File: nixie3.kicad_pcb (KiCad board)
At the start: 2 copper layers, 153 x 96.5 mm, 64 parts, among them J1 AVR-ISP-10, J2 Barrel_Jack, J3 Conn_01x02_Pin, J4 Conn_01x02_Pin, J5 Conn_01x02_Pin, J6 Conn_01x02_Pin, J7 Conn_01x02_Pin, J8 Conn_01x02_Pin, Q1 IRFB4020PBF, U1 ATmega328-A, U2 MCP1401T-E/OT, U3 HV5222PG-G, U4 HV5222PG-G, U5 MC34063AP, Y1 10MHz / 12pF

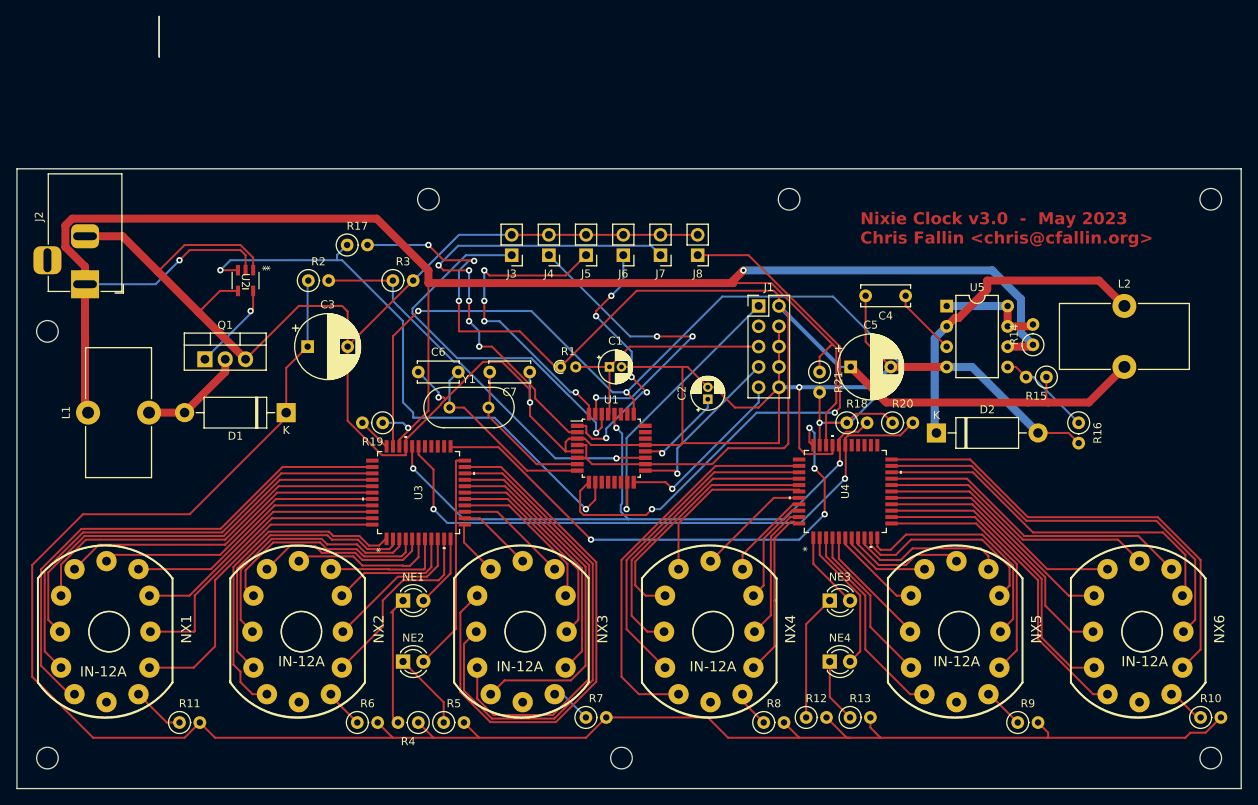
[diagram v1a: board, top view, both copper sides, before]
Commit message: board update
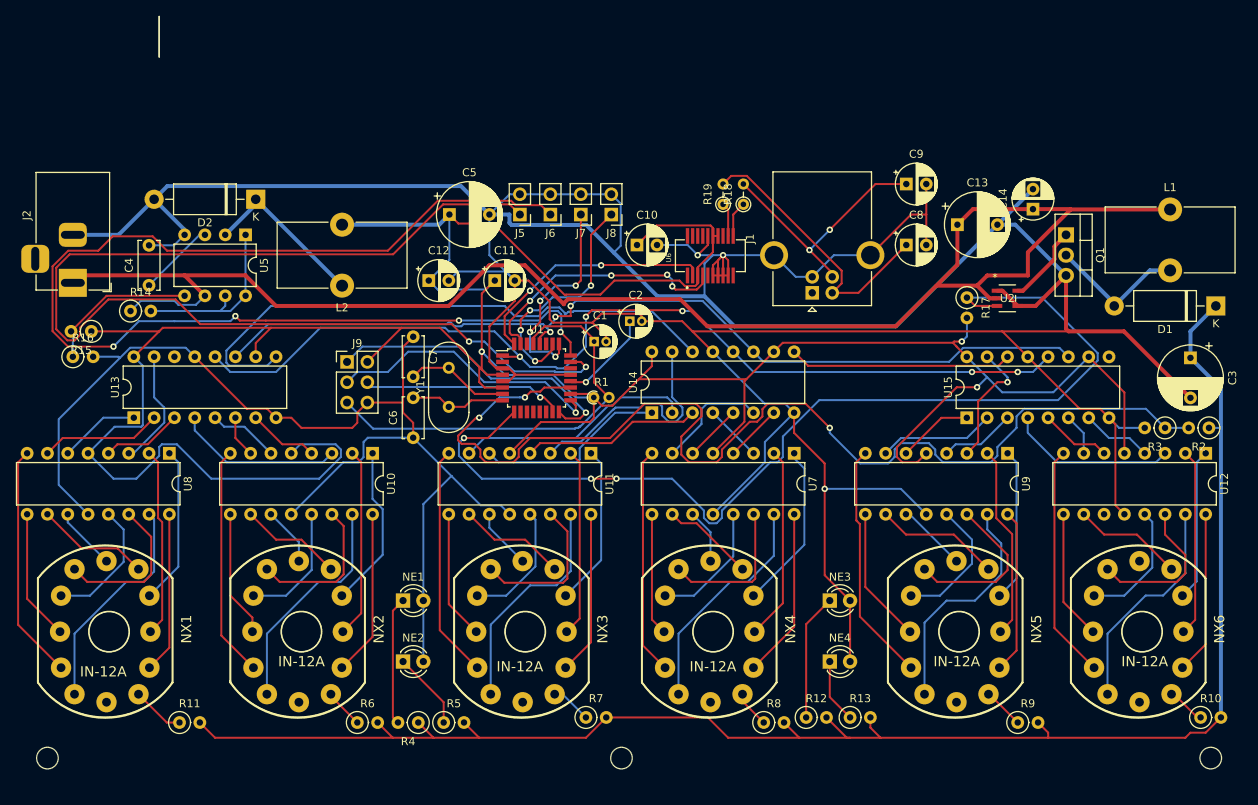
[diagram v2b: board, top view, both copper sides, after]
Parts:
- removed J3, J4: Conn_01x02_Pin, Connector_PinHeader_2.54mm:PinHeader_1x02_P2.54mm_Vertical
- removed R20, R21: 10k, Resistor_THT:R_Axial_DIN0207_L6.3mm_D2.5mm_P2.54mm_Vertical
- removed the REF** at (189.9, 38.7)
- removed the REF** at (44.5, 55.2)
- removed the REF** at (137.2, 38.7)
- removed the REF** at (92.1, 38.7)
- removed U3, U4: HV5222PG-G, import1:QFP44_10x10MC_MCH-M
- added C10: 100nF, Capacitor_THT:CP_Radial_D5.0mm_P2.50mm, F.Cu at (118.2, 44.5)
- added C11: 100nF, Capacitor_THT:CP_Radial_D5.0mm_P2.50mm, F.Cu at (100.4, 48.9)
- added C12: 10uF, Capacitor_THT:CP_Radial_D5.0mm_P2.50mm, F.Cu at (92.1, 48.9)
- added C13: 100uF 25V, Capacitor_THT:CP_Radial_D8.0mm_P5.00mm, F.Cu at (158.2, 41.9)
- added C14: 100nF, Capacitor_THT:CP_Radial_D5.0mm_P2.50mm, F.Cu at (167.6, 40.0)
- added C8: 47pF, Capacitor_THT:CP_Radial_D5.0mm_P2.50mm, F.Cu at (151.8, 44.5)
- added C9: 47pF, Capacitor_THT:CP_Radial_D5.0mm_P2.50mm, F.Cu at (151.8, 36.8)
- added J9: AVR-ISP-6, Connector_PinHeader_2.54mm:PinHeader_2x03_P2.54mm_Vertical, F.Cu at (81.9, 59.1)
- added U10: 74141, Package_DIP:DIP-16_W7.62mm, F.Cu at (85.1, 70.5)
- added U11: 74141, Package_DIP:DIP-16_W7.62mm, F.Cu at (112.4, 70.5)
- added U12: 74141, Package_DIP:DIP-16_W7.62mm, F.Cu at (189.2, 70.5)
- added U13: 74AHC595, Package_DIP:DIP-16_W7.62mm, F.Cu at (55.2, 66.0)
- added U14: 74HC595, Package_DIP:DIP-16_W7.62mm, F.Cu at (120.0, 65.4)
- added U15: 74HC595, Package_DIP:DIP-16_W7.62mm, F.Cu at (159.4, 66.0)
- added U6: FT231XS-R, import3:SOP63P599X175-20N, F.Cu at (127.3, 45.8)
- added U7: 74141, Package_DIP:DIP-16_W7.62mm, F.Cu at (137.8, 70.5)
- added U8: 74141, Package_DIP:DIP-16_W7.62mm, F.Cu at (59.7, 70.5)
- added U9: 74141, Package_DIP:DIP-16_W7.62mm, F.Cu at (164.5, 70.5)
- C3: value C -> 10uF 400V
- J1: value AVR-ISP-10 -> USB_B; footprint Connector_PinHeader_2.54mm:PinHeader_2x05_P2.54mm_Vertical -> Connector_USB:USB_B_OST_USB-B1HSxx_Horizontal
- J2: value Barrel_Jack -> 12V PWR
- R18, R19: value 10k -> 27; footprint Resistor_THT:R_Axial_DIN0207_L6.3mm_D2.5mm_P2.54mm_Vertical -> Resistor_THT:R_Axial_DIN0204_L3.6mm_D1.6mm_P2.54mm_Vertical
- moved L1 137.6 mm to (184.8, 40.0), turned to 0 degrees
- moved R16 126.0 mm to (47.6, 58.4), turned to 0 degrees
- moved R15 119.5 mm to (49.9, 55.2)
- moved D1 117.0 mm to (190.5, 52.1)
- moved R2 114.1 mm to (189.6, 67.3), turned to 180 degrees
- moved R14 112.9 mm to (54.8, 52.7), turned to 0 degrees
- moved C3 110.4 mm to (187.3, 58.6), turned to -90 degrees
- moved Q1 108.8 mm to (171.8, 43.2), turned to -90 degrees
- moved R3 98.3 mm to (184.2, 67.3), turned to 180 degrees
- moved L2 97.8 mm to (81.3, 49.5), turned to 180 degrees
- moved U2 95.3 mm to (164.4, 51.1), turned to 0 degrees
- moved C4 94.6 mm to (57.1, 49.5), turned to 90 degrees
- moved D2 90.0 mm to (70.5, 38.7), turned to 180 degrees
- moved U5 88.1 mm to (69.2, 43.2), turned to -90 degrees
- moved R17 77.7 mm to (159.4, 51.0), turned to -90 degrees
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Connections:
- C1 pad 1: Net-(J1-~{RST}) -> Net-(J9-~{RST})
- J1 pad 1: Net-(J1-MOSI) -> unconnected-(J1-VBUS-Pad1)
- J1 pad 2: VDD -> Net-(J1-D-)
- J1 pad 3: unconnected-(J1-NC-Pad3) -> Net-(J1-D+)
- J1 pad 5: Net-(J1-~{RST}) -> GND
- NE1 pad 2: /Net-(U3A-HVOUT12) -> GND
- NE2 pad 2: /Net-(U3A-HVOUT1) -> GND
- NE3 pad 2: /unconnected-(U4A-HVOUT22-Pad1) -> GND
- NE4 pad 2: /unconnected-(U4A-HVOUT21-Pad2) -> GND
- NX4 pad 0: /unconnected-(U4A-HVOUT23-Pad44) -> Net-(U7-~{Q0})
- NX4 pad 1: /unconnected-(U4A-HVOUT32-Pad35) -> Net-(U7-~{Q1})
- NX4 pad 2: /unconnected-(U4A-HVOUT31-Pad36) -> Net-(U7-~{Q2})
- NX4 pad 3: /unconnected-(U4A-HVOUT30-Pad37) -> Net-(U7-~{Q3})
- NX4 pad 4: /unconnected-(U4A-HVOUT29-Pad38) -> Net-(U7-~{Q4})
- NX4 pad 5: /unconnected-(U4A-HVOUT28-Pad39) -> Net-(U7-~{Q5})
- NX4 pad 6: /unconnected-(U4A-HVOUT27-Pad40) -> Net-(U7-~{Q6})
- NX4 pad 7: /unconnected-(U4A-HVOUT26-Pad41) -> Net-(U7-~{Q7})
- NX4 pad 8: /unconnected-(U4A-HVOUT25-Pad42) -> Net-(U7-~{Q8})
- NX4 pad 9: /unconnected-(U4A-HVOUT24-Pad43) -> Net-(U7-~{Q9})
- NX5 pad 0: /unconnected-(U4A-HVOUT11-Pad12) -> Net-(U9-~{Q0})
- NX5 pad 1: /unconnected-(U4A-HVOUT20-Pad3) -> Net-(U9-~{Q1})
- NX5 pad 2: /unconnected-(U4A-HVOUT19-Pad4) -> Net-(U9-~{Q2})
- NX5 pad 3: /unconnected-(U4A-HVOUT18-Pad5) -> Net-(U9-~{Q3})
- NX5 pad 4: /unconnected-(U4A-HVOUT17-Pad6) -> Net-(U9-~{Q4})
- NX5 pad 5: /unconnected-(U4A-HVOUT16-Pad7) -> Net-(U9-~{Q5})
- NX5 pad 6: /unconnected-(U4A-HVOUT15-Pad8) -> Net-(U9-~{Q6})
- NX5 pad 7: /unconnected-(U4A-HVOUT14-Pad9) -> Net-(U9-~{Q7})
- NX5 pad 8: /unconnected-(U4A-HVOUT13-Pad10) -> Net-(U9-~{Q8})
- NX5 pad 9: /unconnected-(U4A-HVOUT12-Pad11) -> Net-(U9-~{Q9})
- NX6 pad 0: /unconnected-(U4A-HVOUT1-Pad22) -> Net-(U12-~{Q0})
- NX6 pad 1: /unconnected-(U4A-HVOUT10-Pad13) -> Net-(U12-~{Q1})
- NX6 pad 2: /unconnected-(U4A-HVOUT9-Pad14) -> Net-(U12-~{Q2})
- NX6 pad 3: /unconnected-(U4A-HVOUT8-Pad15) -> Net-(U12-~{Q3})
- NX6 pad 4: /unconnected-(U4A-HVOUT7-Pad16) -> Net-(U12-~{Q4})
- NX6 pad 5: /unconnected-(U4A-HVOUT6-Pad17) -> Net-(U12-~{Q5})
- NX6 pad 6: /unconnected-(U4A-HVOUT5-Pad18) -> Net-(U12-~{Q6})
- NX6 pad 7: /unconnected-(U4A-HVOUT4-Pad19) -> Net-(U12-~{Q7})
- NX6 pad 8: /unconnected-(U4A-HVOUT3-Pad20) -> Net-(U12-~{Q8})
- NX6 pad 9: /unconnected-(U4A-HVOUT2-Pad21) -> Net-(U12-~{Q9})
- R1 pad 2: Net-(J1-~{RST}) -> Net-(J9-~{RST})
- R17 pad 1: Net-(U1-PD6) -> Net-(U1-PD5)
- R18 pad 1: VCC -> Net-(U6-USBDP)
- R18 pad 2: Net-(U1-PC5) -> Net-(J1-D+)
- R19 pad 1: VCC -> Net-(U6-USBDM)
- R19 pad 2: Net-(U3A-DATAIN) -> Net-(J1-D-)
- U1 pad 1: Net-(J6-Pin_1) -> Net-(U1-PD3)
- U1 pad 10: Net-(U1-PD6) -> unconnected-(U1-PD6-Pad10)
- U1 pad 15: Net-(J1-MOSI) -> Net-(J9-MOSI)
- U1 pad 16: Net-(J1-MISO) -> Net-(J9-MISO)
- U1 pad 17: Net-(J1-SCK) -> Net-(J9-SCK)
- U1 pad 2: Net-(J7-Pin_1) -> unconnected-(U1-PD4-Pad2)
- U1 pad 23: unconnected-(U1-PC0-Pad23) -> Net-(J5-Pin_1)
- U1 pad 24: unconnected-(U1-PC1-Pad24) -> Net-(J6-Pin_1)
- U1 pad 25: Net-(U1-PC2) -> Net-(J7-Pin_1)
- U1 pad 26: unconnected-(U1-PC3-Pad26) -> Net-(J8-Pin_1)
- U1 pad 27: unconnected-(U1-PC4-Pad27) -> Net-(U1-PC4)
- U1 pad 29: Net-(J1-~{RST}) -> Net-(J9-~{RST})
- U1 pad 32: Net-(J5-Pin_1) -> Net-(U1-PD2)
- U1 pad 9: Net-(J8-Pin_1) -> Net-(U1-PD5)
- U2 pad 3: Net-(U1-PD6) -> Net-(U1-PD5)
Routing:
- net GND: track 320.2 -> 671.1 mm
- net VDD: track 173.3 -> 396.0 mm
- net Net-(U1-PD5): track 0.00 -> 128.8 mm, vias 0 -> 3
- net Net-(U1-PD3): track 0.00 -> 120.8 mm, vias 0 -> 5
- net Net-(U1-PC2): track 114.8 -> 0.00 mm, vias 3 -> 0
- net Net-(J6-Pin_1): track 34.1 -> 148.5 mm, vias 5 -> 4
- net Net-(J5-Pin_1): track 38.9 -> 145.1 mm, vias 4 -> 2
- net Net-(U1-ADC6): track 50.4 -> 139.4 mm, vias 1 -> 3
- net Net-(U3A-OE): track 77.2 -> 0.00 mm, vias 2 -> 0
- net Net-(U1-PD6): track 73.9 -> 0.00 mm, vias 2 -> 0
- net Net-(U13-QH'): track 0.00 -> 72.8 mm
- net Net-(U3A-DATAOUT): track 66.9 -> 0.00 mm, vias 4 -> 0
- net VCC: track 252.4 -> 193.7 mm, vias 3 -> 0
- net /unconnected-(U4A-HVOUT1-Pad22): track 58.3 -> 0.00 mm
- net Net-(U11-~{Q4}): track 70.0 -> 15.6 mm
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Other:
- board outline removed
- board text removed: "Nixie Clock v3.0 - May 2023 Chris Fallin <chris@cfallin.org>"
